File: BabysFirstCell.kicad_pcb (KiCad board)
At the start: 4 copper layers, 56.4 x 56.4 mm, 18 parts, among them J1 Uart vcc gnd rx tx, J2 Head, J3 Conn_01x05, U2 MCP1703Ax-330xxTT, U3 STM32G051F8Px

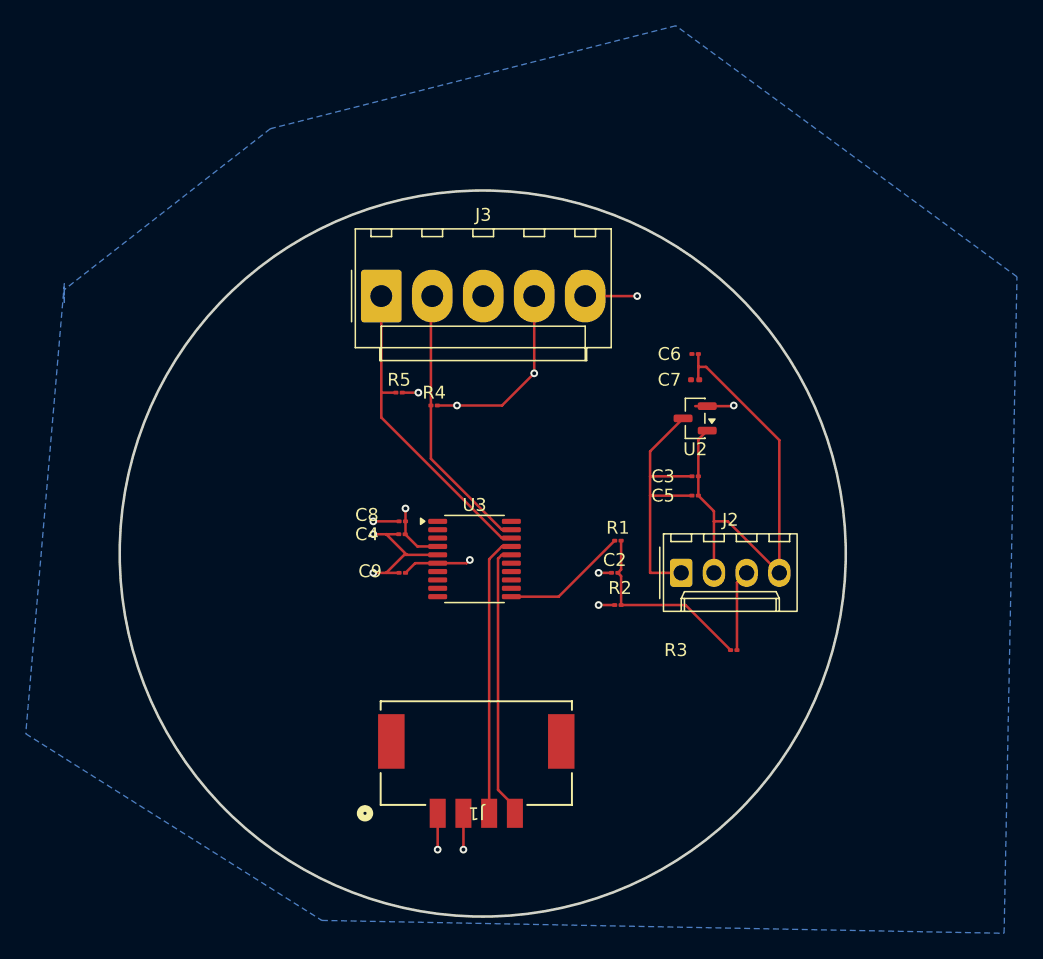
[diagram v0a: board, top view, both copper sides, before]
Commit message: Add EasyEDA Pro project files
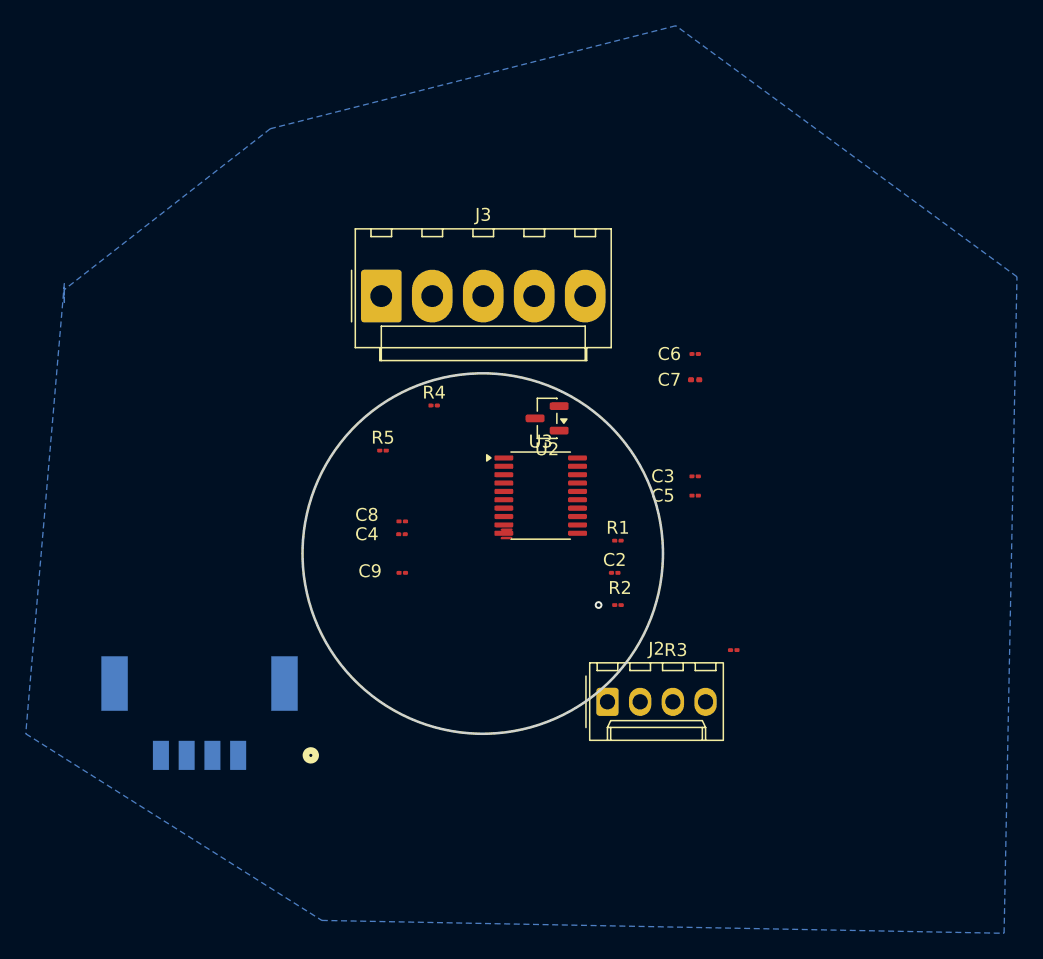
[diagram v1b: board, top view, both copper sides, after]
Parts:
- J1: moved to B.Cu
- moved J1 22.0 mm to (123.0, 105.5), turned to 0 degrees
- moved J2 11.5 mm to (154.7, 106.0)
- moved U2 11.5 mm to (150.0, 84.0)
- moved U3 7.12 mm to (149.5, 90.0)
- moved R5 4.67 mm to (137.2, 86.5)
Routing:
- net GND: track 72.1 -> 0.10 mm, vias 8 -> 1
- net Net-(J3-Pin_3): track 26.3 -> 0.00 mm, vias 1 -> 0
- net /SWDIO: track 24.5 -> 0.74 mm
- net +7.5V: track 22.0 -> 0.00 mm
- net Net-(J1-Pin_3): track 21.9 -> 0.00 mm
- net Net-(J1-Pin_4): track 21.5 -> 0.00 mm
- net Net-(J3-Pin_2): track 21.2 -> 0.15 mm
- net +3.3V: track 16.1 -> 0.04 mm, vias 5 -> 0
- net Net-(C2-Pad2): track 15.2 -> 0.00 mm
- net Net-(U3-PA4): track 9.83 -> 0.00 mm
- net Net-(J2-Pin_3): track 6.31 -> 0.00 mm
- net unconnected-(U3-PA3-Pad10): track 0.00 -> 0.74 mm
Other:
- board size 56.4 x 56.4 mm -> 28 x 28 mm
